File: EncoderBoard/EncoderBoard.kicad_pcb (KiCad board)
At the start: 2 copper layers, 221 x 61 mm, 222 parts, among them SW1 Rotary_Encoder_Switch, SW10 SW_Push_LED_Red, SW11 SW_Push_LED_Blue, SW12 SW_Push_LED_Red, SW13 SW_Push_LED_Yellow, SW14 SW_Push_LED_Green, SW15 SW_Push_LED_Blue, SW2 Rotary_Encoder_Switch, SW3 Rotary_Encoder_Switch, SW4 Rotary_Encoder_Switch, SW5 Rotary_Encoder_Switch, SW6 Rotary_Encoder_Switch, SW7 Rotary_Encoder_Switch, SW8 Rotary_Encoder_Switch, SW9 Rotary_Encoder_Switch, U1 MCP23S17_SO, U10 Display_OLED_128x32_I2C, U11 Display_OLED_128x32_I2C, U12 Display_OLED_128x32_I2C, U13 Display_OLED_128x32_I2C, U14 Display_OLED_128x32_I2C, U15 Display_OLED_128x32_I2C, U16 Display_OLED_128x32_I2C, U17 Display_OLED_128x32_I2C, U18 74LVC14, U19 74LCV14, U2 MCP23S17_SO, U20 74LVC14, U21 74LVC14, U22 74LVC14, U23 74LVC14, U24 CAT24M01W, U25 CAT24M01W, U26 CAT24M01W, U3 MCP23S17_SO, U4 TCA9548APWR, U5 74HCT245, U6 TCA9548APWR, U7 Teensy3.2, U8 CAT24M01W, U9 Display_OLED_128x32_I2C

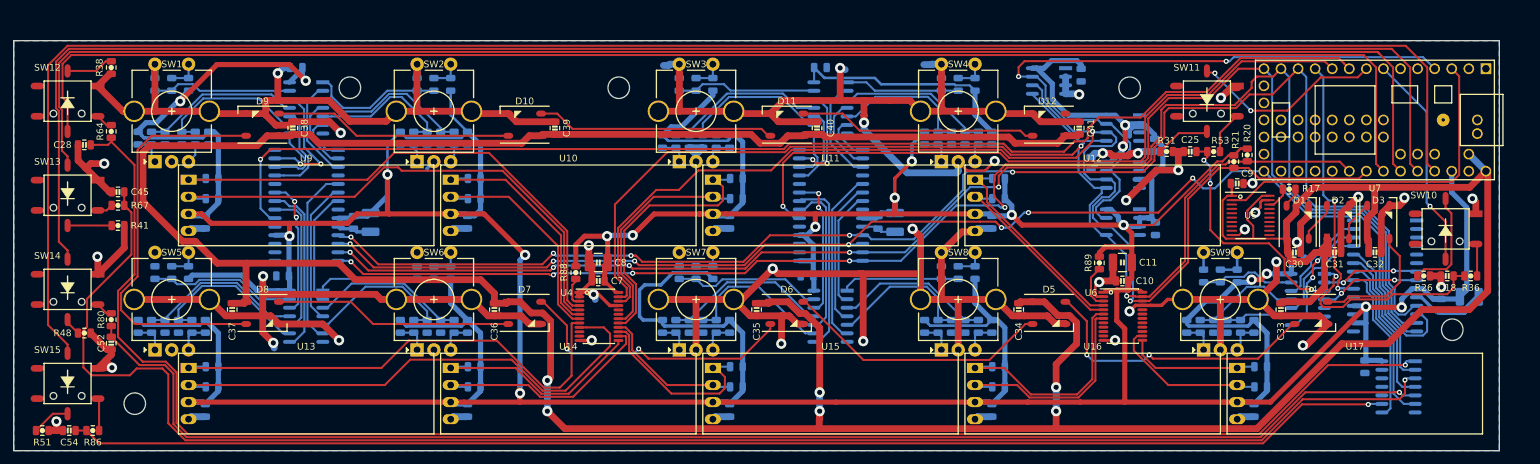
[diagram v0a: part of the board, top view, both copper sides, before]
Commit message: Small changes.
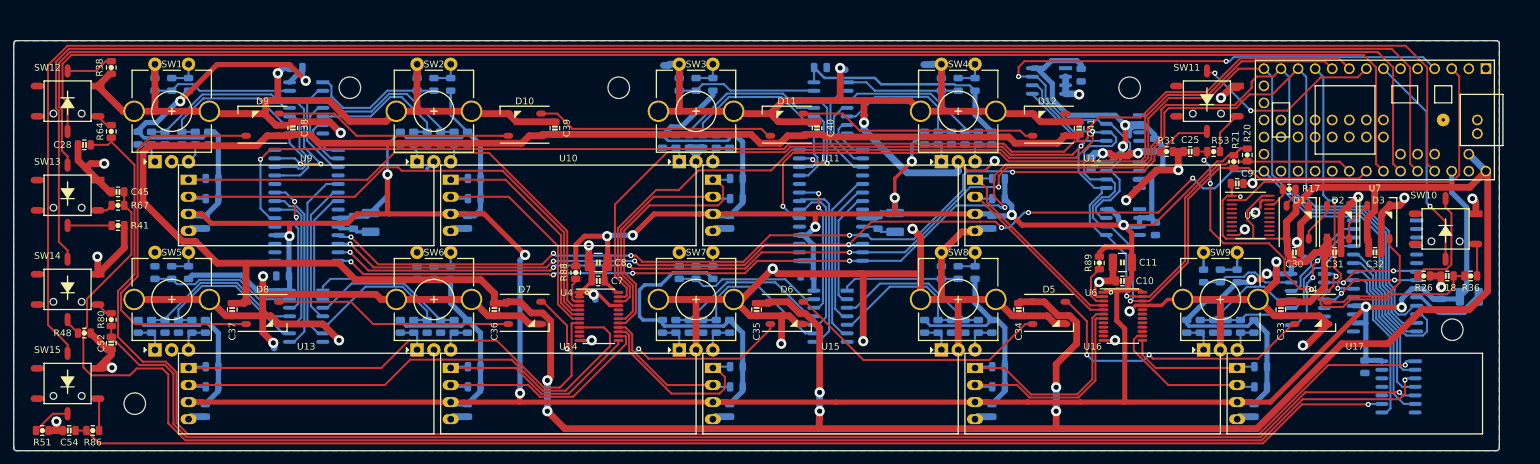
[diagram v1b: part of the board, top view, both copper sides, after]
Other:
- outline, holes or cut-outs redrawn
